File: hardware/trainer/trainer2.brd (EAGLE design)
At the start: 86 x 56 mm, 53 parts, among them Q1 2N3906, Q2 2N3906, Q3 2N3906, Q4 2N3906

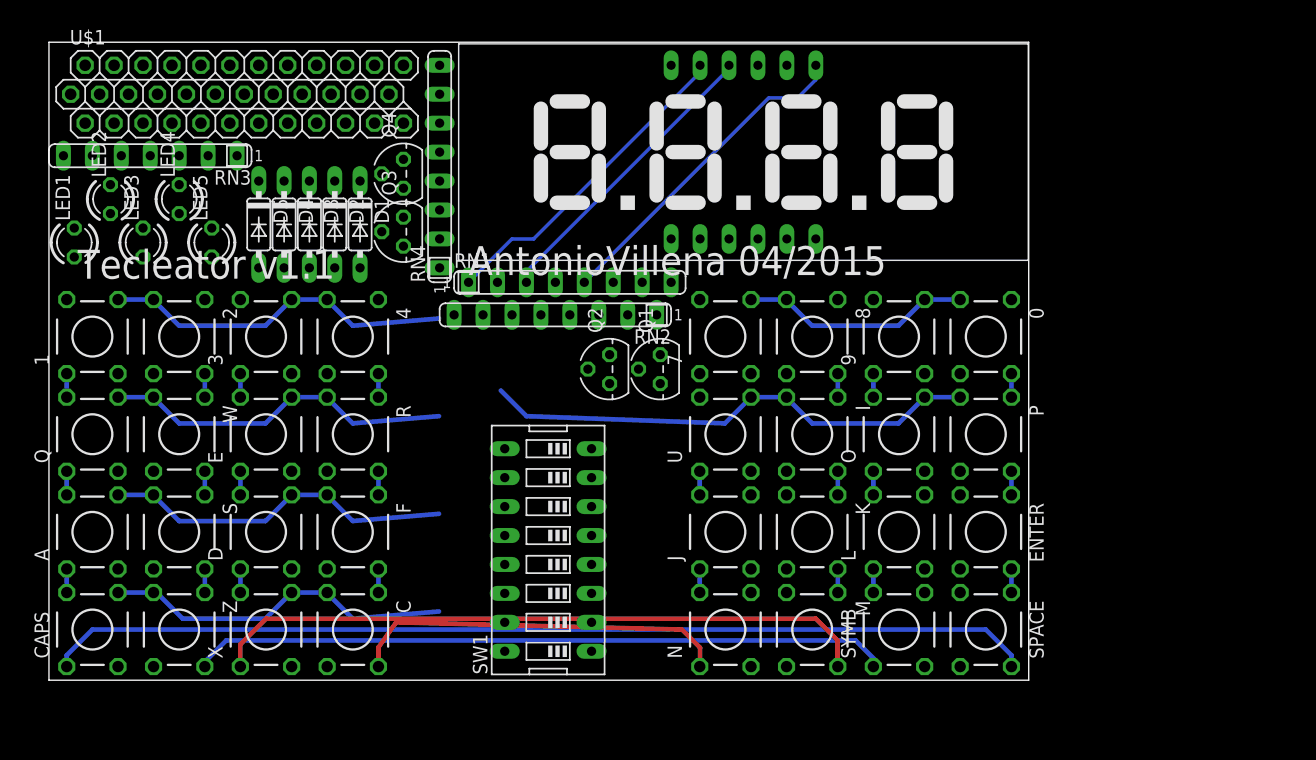
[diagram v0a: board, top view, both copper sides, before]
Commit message: Añado trainer2
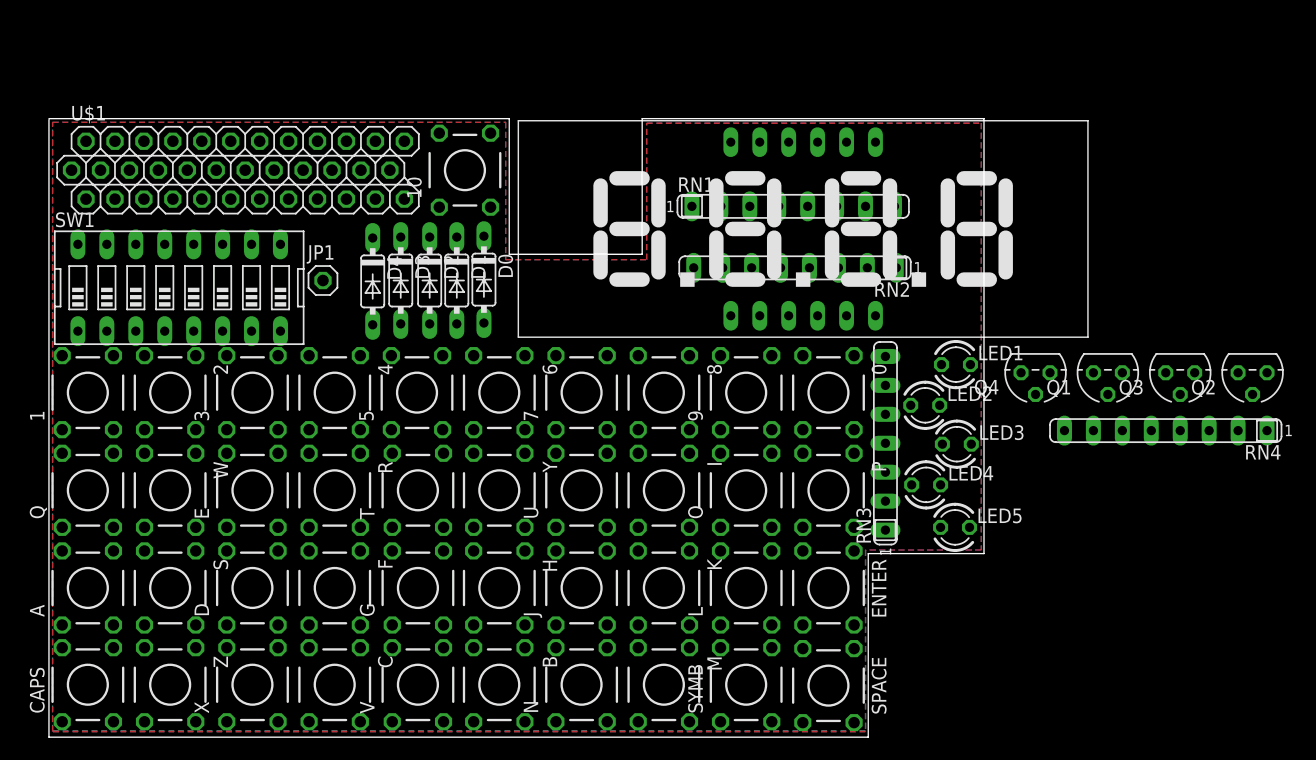
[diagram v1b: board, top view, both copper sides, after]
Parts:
- removed D5: 1N4148DO35-7, diode:DO35-7
- added 10, 5, 6, B, G, H, T, V, Y: (no value), switch-tact:DTS-6
- added D0: (no value), diode:DO35-7
- added JP1: (no value), pinhead:1X01
- D1, D2, D3, D4: value 1N4148DO35-7 -> (none)
- RN1, RN2: value 2K2 -> 100
- RN4: value (none) -> 2K2
- moved LED1 78.1 mm to (79.6, 27.7), turned to 0 degrees
- moved LED2 73.8 mm to (76.9, 24.1), turned to 0 degrees
- moved LED3 73.6 mm to (79.7, 20.7), turned to 0 degrees
- moved LED4 70.2 mm to (77.0, 17.1), turned to 0 degrees
- moved LED5 69.9 mm to (79.5, 13.4), turned to 0 degrees
- moved Q3 69.3 mm to (99.3, 27.0), turned to 180 degrees
- moved RN3 69.3 mm to (73.4, 20.8), turned to 90 degrees
- moved RN4 67.8 mm to (98.0, 21.9), turned to 180 degrees
- moved Q4 58.2 mm to (86.6, 27.0), turned to 180 degrees
- moved Q2 56.4 mm to (105.6, 27.0), turned to 180 degrees
- moved SW1 39.7 mm to (11.4, 34.4), turned to 0 degrees
- moved Q1 39.3 mm to (92.9, 27.0), turned to 180 degrees
- moved RN2 21.4 mm to (65.5, 36.2)
- moved RN1 20.7 mm to (65.3, 41.6)
- moved 0 14.7 mm to (68.4, 25.2)
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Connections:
- removed net N$33 (its old number): RN2.7, U$2.4
- removed net N$34 (its old number): RN2.5, U$2.2
- removed net N$35 (its old number): RN2.1, U$2.1
- removed net N$36 (its old number): RN1.3, U$2.10
- new net N$11: RN1.5, U$2.4
- new net N$12: RN2.7, U$2.2
- new net N$13: RN2.5, U$2.1
- new net N$14: RN2.1, U$2.10
- new net N$15: 10.3, JP1.1
- new net N$28: B.2, V.1
- new net N$29: 5.1, T.2
- new net N$40: 7.1, U.2
- new net N$42: G.1, V.2
- new net N$45: SW1.1, SW1.2, SW1.3, SW1.4, SW1.5, SW1.6, SW1.7, SW1.8
- new net N$50: B.1, H.2
- new net N$51: H.1, Y.2
- new net N$55: 6.2, Y.1
- new net N$56: 9.1, O.2
- net A10: now also SW1.14, T.4; no longer SW1.10
- net A11: now also 5.4, SW1.13; no longer SW1.9
- net A12: now also 6.3, SW1.12; no longer SW1.4
- net A13: now also SW1.11, Y.3; no longer SW1.3
- net A14: now also H.3, SW1.10; no longer SW1.2
- net A15: now also B.3, SW1.9; no longer SW1.1
- net A8: now also SW1.16, V.4; no longer SW1.12
- net A9: now also G.4, SW1.15; no longer SW1.11
- net D0: now also D0.A; no longer D5.A
- net D1: now also D1.A; no longer 9.1, D4.A, O.2
- net D2: now also D2.A; no longer D3.A
- net D3: now also D3.A; no longer D2.A
- net D4: now also 5.2, D4.A; no longer D1.A, SW1.13, SW1.14, SW1.15, SW1.16, SW1.5, SW1.6, SW1.7, SW1.8
- net DIG1: now also U$1.P19; no longer U$1.P18
- net DIG3: now also U$1.P18; no longer U$1.P17
- net DIG4: now also U$1.P23; no longer U$1.P26
- net DISB: now also RN1.4; no longer RN1.6
- net DISC: now also RN1.6; no longer RN2.8
- net DISD: now also U$1.P33; no longer U$1.P34
- net DISDP: now also RN2.8, U$1.P6; no longer RN2.2, U$1.P10
- net DISE: now also RN2.2; no longer RN1.4
- net DISF: now also U$1.P17; no longer U$1.P19
- net DISG: now also U$1.P12; no longer U$1.P15
- net GND: now also 10.1
- net LED1: no longer U$1.P35
- net LED2: no longer U$1.P32
- net LED3: now also U$1.P32; no longer U$1.P33
- net LED4: now also U$1.P26; no longer U$1.P23
- net LED6: now also U$1.P24; no longer U$1.P20
- net N$10: now also RN1.3, U$2.7; no longer 7.2, U.2
- net N$30: now also G.2, T.1; no longer RN1.5, U$2.7
- net PUSH2: now also U$1.P20; no longer U$1.P24
- net SW1: now also U$1.P9; no longer U$1.P6
- net SW4: now also U$1.P11; no longer U$1.P9
- net SW5: now also U$1.P10; no longer U$1.P11
- net SW6: now also U$1.P14; no longer U$1.P12
- net SW7: now also U$1.P15; no longer U$1.P14
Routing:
- net N$22: track 86.8 -> 0.00 mm
- net N$19: track 61.5 -> 0.00 mm
- net ELETE: track 58.4 -> 0.00 mm
- net A13: track 44.1 -> 0.00 mm
- net N$43: track 33.4 -> 0.00 mm
- net A11: track 31.1 -> 0.00 mm
- net A8: track 31.1 -> 0.00 mm
- net A10: track 31.1 -> 0.00 mm
- net A9: track 31.1 -> 0.00 mm
- net N$30: track 29.0 -> 0.00 mm
- net N$9: track 28.6 -> 0.00 mm
- net N$36 (its old number): track 26.4 -> 0.00 mm
- net A12: track 20.3 -> 0.00 mm
- net N$54: track 2.07 -> 0.00 mm
- net N$53: track 2.07 -> 0.00 mm
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- added copper zone on layer 1, net GND
- added copper zone on layer 16, net GND
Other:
- board size 86 x 56 mm -> 82.1 x 54.3 mm
- board text removed: "AntonioVillena 04/2015"
- board text removed: "Tecleator v1.1"
